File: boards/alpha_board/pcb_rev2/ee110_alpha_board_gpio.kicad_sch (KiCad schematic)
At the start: 37 parts, among them J4 keypad, J5 Micro_SD_Card, J6 SERVO1, J7 SERVO2, U5 74LS138, U6 74LVC245, U7 LM386, U8 LM2902, U9 MPU-9250

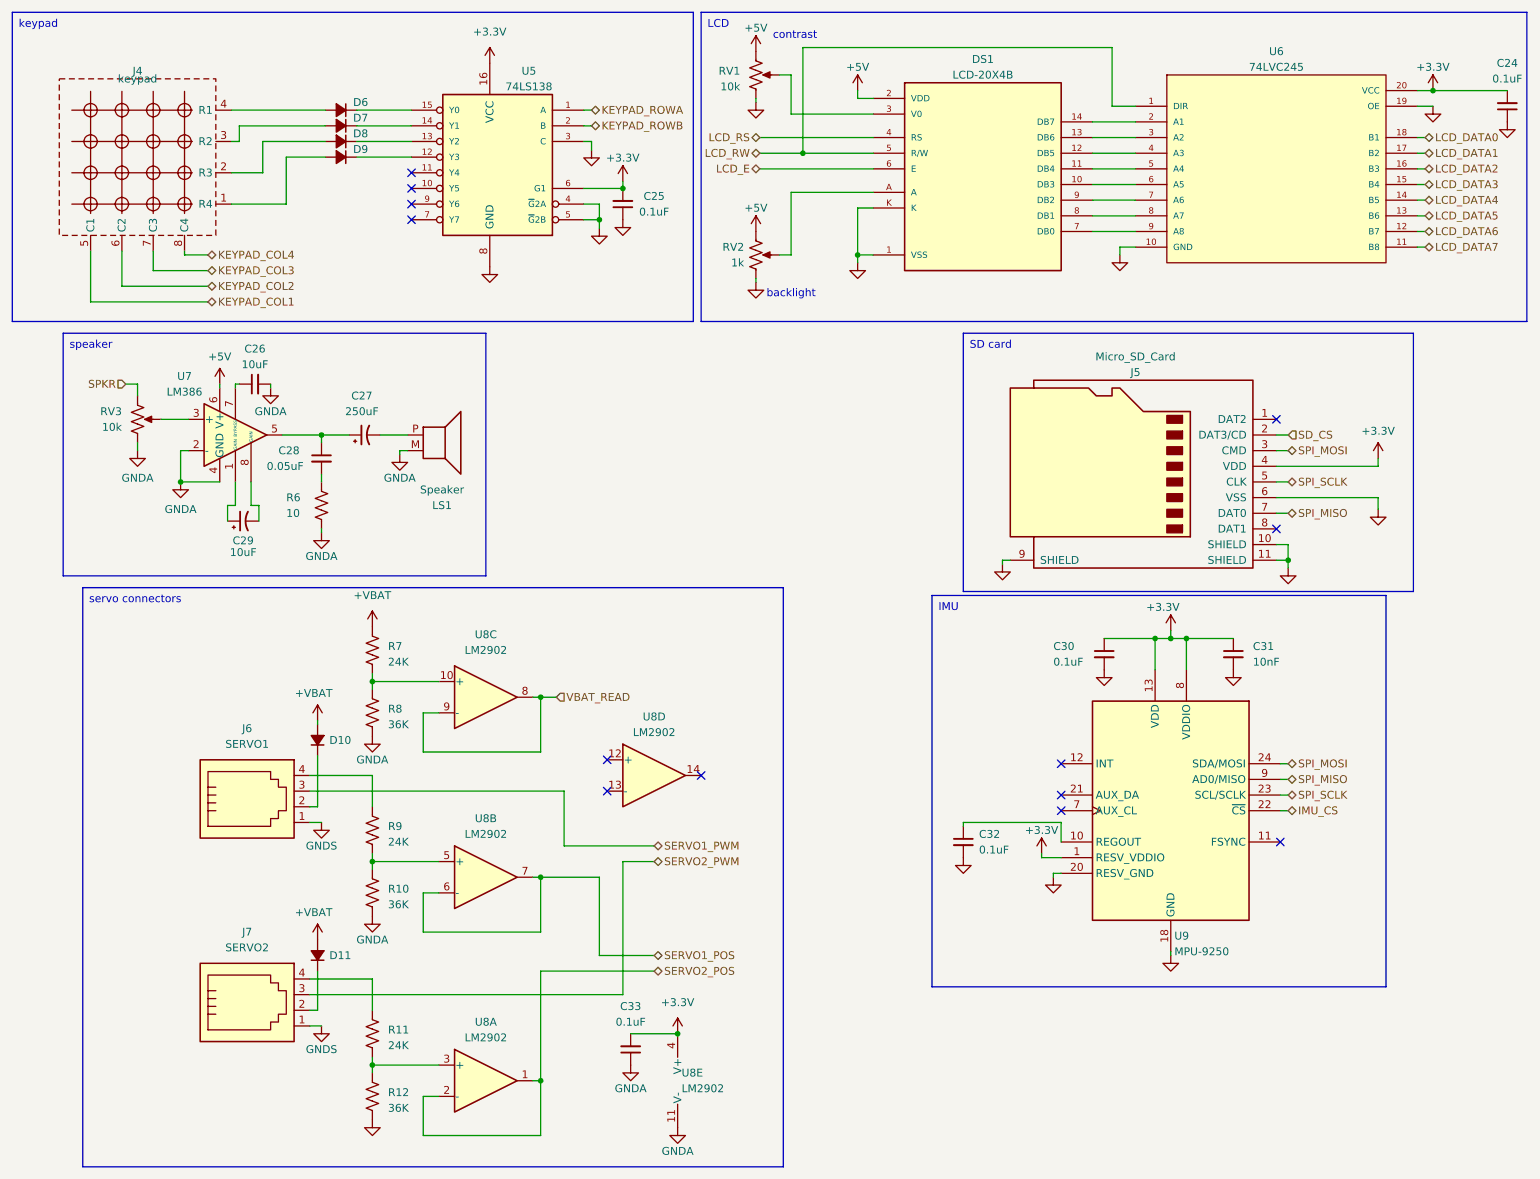
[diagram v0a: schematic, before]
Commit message: 4/27
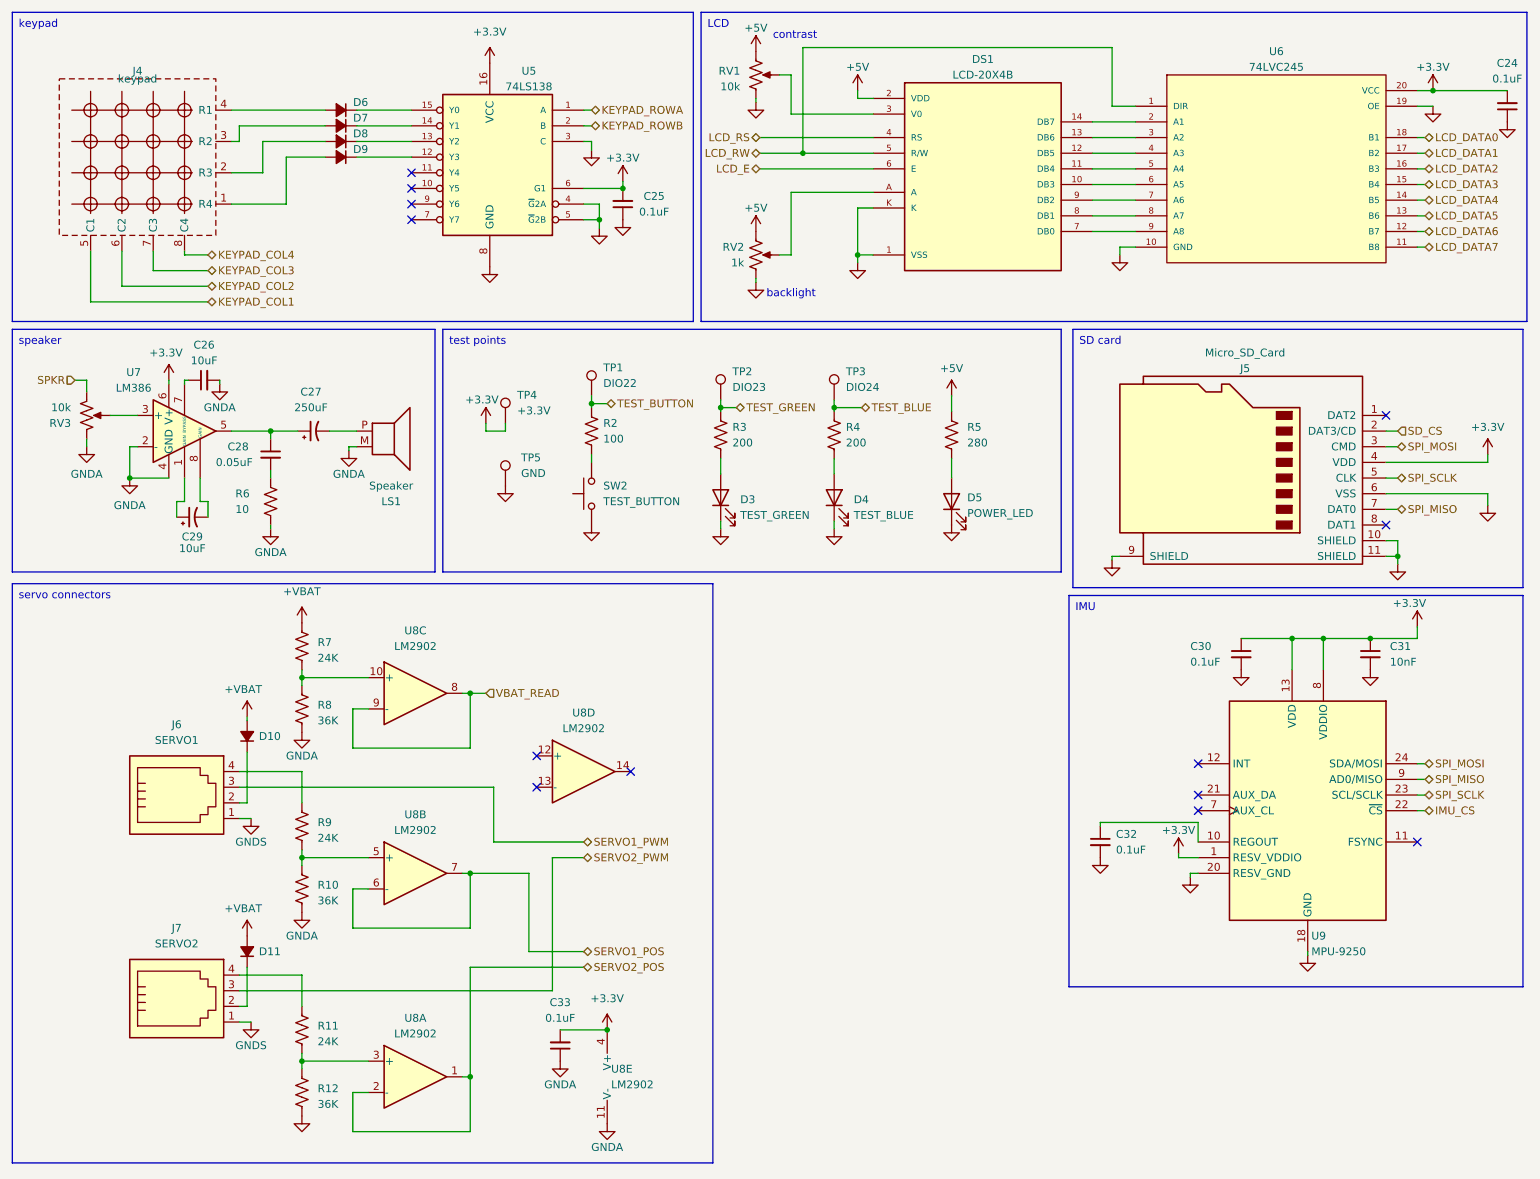
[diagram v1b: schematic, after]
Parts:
- added D3: TEST_GREEN, LED_SMD:LED_0805_2012Metric_Pad1.15x1.40mm_HandSolder, symbol Device:LED
- added D4: TEST_BLUE, LED_SMD:LED_0805_2012Metric_Pad1.15x1.40mm_HandSolder, symbol Device:LED
- added D5: POWER_LED, LED_THT:LED_D3.0mm, symbol Device:LED
- added R2: 100, Resistor_SMD:R_0805_2012Metric_Pad1.20x1.40mm_HandSolder, symbol Device:R_US
- added R3, R4: 200, Resistor_SMD:R_0805_2012Metric_Pad1.20x1.40mm_HandSolder, symbol Device:R_US
- added R5: 280, Resistor_SMD:R_0805_2012Metric_Pad1.20x1.40mm_HandSolder, symbol Device:R_US
- added SW2: TEST_BUTTON, Button_Switch_SMD:SW_SPST_TL3342, symbol Switch:SW_Push
- added TP1: DIO22, TestPoint:TestPoint_THTPad_2.0x2.0mm_Drill1.0mm, symbol Connector:TestPoint
- added TP2: DIO23, TestPoint:TestPoint_THTPad_2.0x2.0mm_Drill1.0mm, symbol Connector:TestPoint
- added TP3: DIO24, TestPoint:TestPoint_THTPad_2.0x2.0mm_Drill1.0mm, symbol Connector:TestPoint
- added TP4: +3.3V, TestPoint:TestPoint_THTPad_2.0x2.0mm_Drill1.0mm, symbol Connector:TestPoint
- added TP5: GND, TestPoint:TestPoint_THTPad_2.0x2.0mm_Drill1.0mm, symbol Connector:TestPoint
- U9: footprint Package_DFN_QFN:QFN-24-1EP_3x3mm_P0.4mm_EP1.75x1.6mm -> Alpha Board rev2 library:QFN-24-1EP_3x3mm_P0.4mm_EP1.75x1.6mm
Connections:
- net +3.3V: now also U7.6 (V+), TP4.1
- net +5V: now also R5.1; no longer U7.6 (V+)
- net GND: now also D3.1 (K), D4.1 (K), D5.1 (K), SW2.1, TP5.1
- net GNDA: now also RV3.1; no longer RV3.3
- net SPKR: now also RV3.3; no longer RV3.1
- new net: R2.1, SW2.2
- new net: D3.2 (A), R3.1
- new net: D5.2 (A), R5.2
- new net: D4.2 (A), R4.1
- new net TEST_BLUE: R4.2, TP3.1
- new net TEST_BUTTON: R2.2, TP1.1
- new net TEST_GREEN: R3.2, TP2.1
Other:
- moved on the sheet: C26, C27, C28, C29, C30, C31, C32, C33, D10, D11, J5, J6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
